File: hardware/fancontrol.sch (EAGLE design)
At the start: 7 parts, among them Q1 IRLZ44Z, T1 BC547

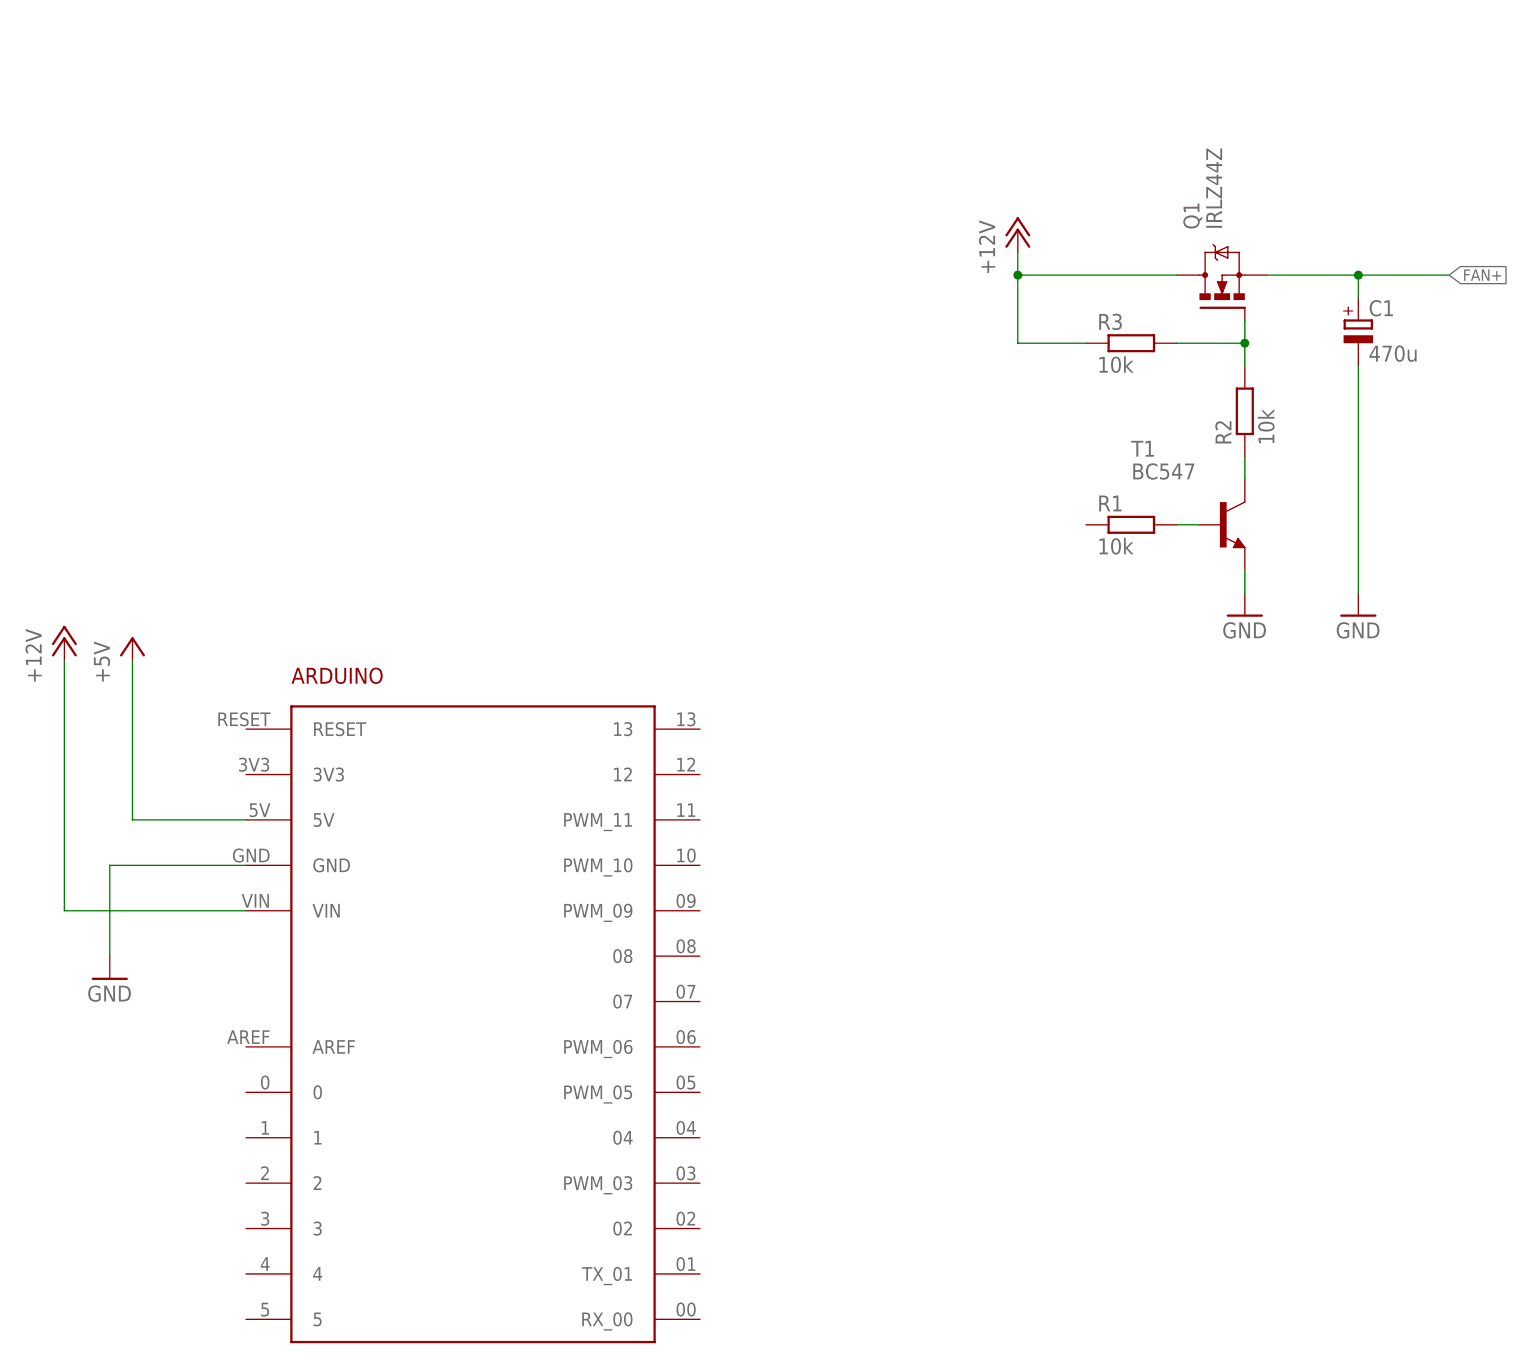
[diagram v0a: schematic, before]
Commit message: generated board
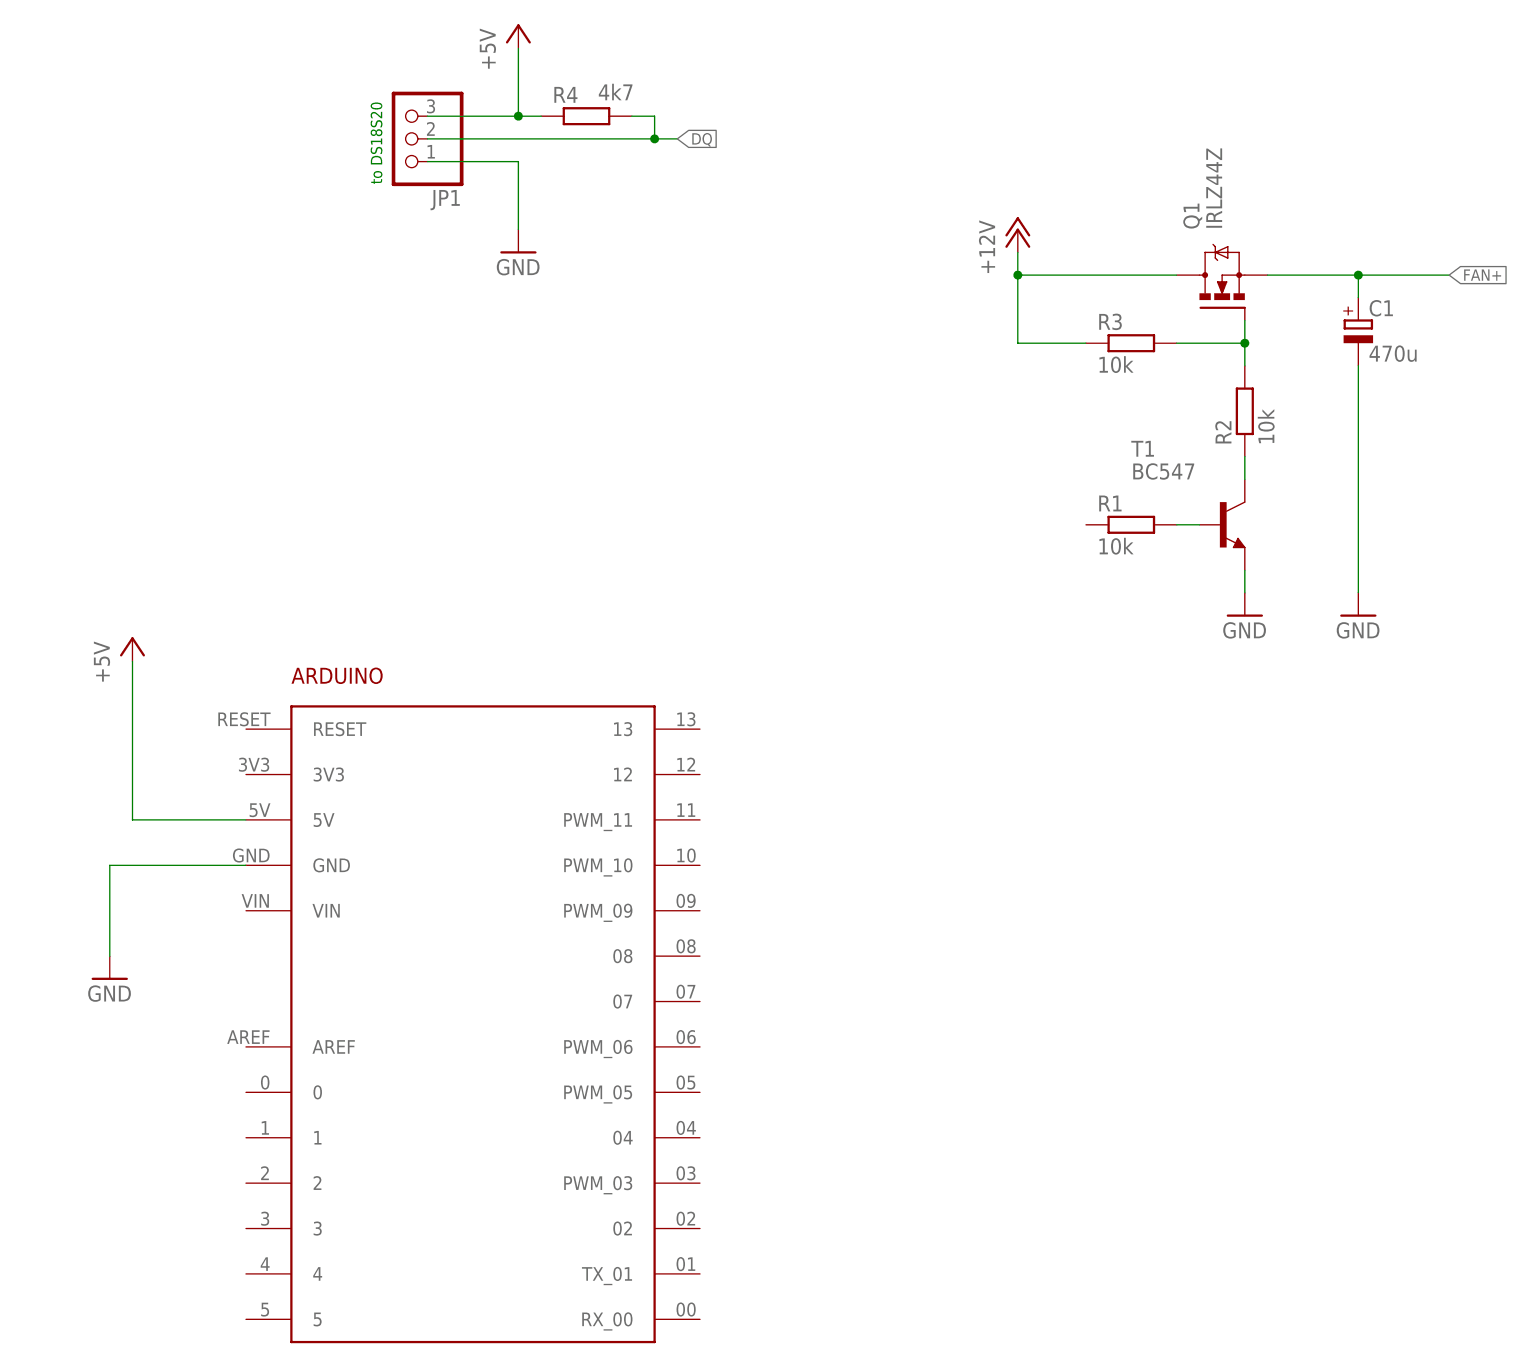
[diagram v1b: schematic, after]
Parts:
- added JP1: (no value), pinhead:PINHD-1X3
- added R4: 4k7, rcl:R-EU_0207/7
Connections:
- new net DQ: JP1.2, R4.2
- net +12V: no longer ARDUINO1.VIN
- net +5V: now also JP1.3, R4.1
- net GND: now also JP1.1
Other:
- note added: "to DS18S20"
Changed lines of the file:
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@@
 <part name="ARDUINO1" library="arduino" deviceset="ARDUINO" device=""/>
 <part name="GND3" library="supply1" deviceset="GND" device=""/>
-<part name="P+3" library="supply1" deviceset="+12V" device=""/>
 <part name="P+4" library="supply1" deviceset="+5V" device=""/>
+<part name="JP1" library="pinhead" deviceset="PINHD-1X3" device=""/>
+<part name="P+1" library="supply1" deviceset="+5V" device=""/>
+<part name="GND4" library="supply1" deviceset="GND" device=""/>
+<part name="R4" library="rcl" deviceset="R-EU_" device="0207/7" value="4k7"/>
 </parts>
 <sheets>
 <sheet>
 <plain>
+<text x="40.64" y="142.24" size="1.27" layer="91" rot="R90">to DS18S20</text>
 </plain>
 <instances>
@@
 <instance part="ARDUINO1" gate="G$1" x="50.8" y="50.8"/>
 <instance part="GND3" gate="1" x="10.16" y="53.34"/>
-<instance part="P+3" gate="1" x="5.08" y="91.44"/>
 <instance part="P+4" gate="1" x="12.7" y="91.44"/>
+<instance part="JP1" gate="A" x="43.18" y="147.32" rot="R180"/>
+<instance part="P+1" gate="1" x="55.88" y="160.02"/>
+<instance part="GND4" gate="1" x="55.88" y="134.62"/>
+<instance part="R4" gate="G$1" x="63.5" y="149.86" smashed="yes">
+<attribute name="NAME" x="59.69" y="151.3586" size="1.778" layer="95"/>
+<attribute name="VALUE" x="64.77" y="151.638" size="1.778" layer="96"/>
+</instance>
 </instances>
 <busses>
@@
 <wire x1="10.16" y1="66.04" x2="10.16" y2="55.88" width="0.1524" layer="91"/>
 </segment>
+<segment>
+<pinref part="JP1" gate="A" pin="1"/>
+<pinref part="GND4" gate="1" pin="GND"/>
+<wire x1="45.72" y1="144.78" x2="55.88" y2="144.78" width="0.1524" layer="91"/>
+<wire x1="55.88" y1="144.78" x2="55.88" y2="137.16" width="0.1524" layer="91"/>
+</segment>
 </net>
 <net name="N$3" class="0">
@@
 <junction x="111.76" y="132.08"/>
 </segment>
-<segment>
-<pinref part="ARDUINO1" gate="G$1" pin="VIN"/>
-<pinref part="P+3" gate="1" pin="+12V"/>
-<wire x1="25.4" y1="60.96" x2="5.08" y2="60.96" width="0.1524" layer="91"/>
-<wire x1="5.08" y1="60.96" x2="5.08" y2="88.9" width="0.1524" layer="91"/>
-</segment>
 </net>
 <net name="FAN+" class="0">
@@
 <wire x1="12.7" y1="71.12" x2="12.7" y2="88.9" width="0.1524" layer="91"/>
 </segment>
+<segment>
+<pinref part="JP1" gate="A" pin="3"/>
+<pinref part="R4" gate="G$1" pin="1"/>
+<wire x1="45.72" y1="149.86" x2="55.88" y2="149.86" width="0.1524" layer="91"/>
+<pinref part="P+1" gate="1" pin="+5V"/>
+<wire x1="55.88" y1="149.86" x2="58.42" y2="149.86" width="0.1524" layer="91"/>
+<wire x1="55.88" y1="157.48" x2="55.88" y2="149.86" width="0.1524" layer="91"/>
+<junction x="55.88" y="149.86"/>
+</segment>
 </net>
+<net name="DQ" class="0">
+<segment>
+<pinref part="JP1" gate="A" pin="2"/>
+<wire x1="45.72" y1="147.32" x2="71.12" y2="147.32" width="0.1524" layer="91"/>
+<label x="73.66" y="147.32" size="1.27" layer="95" xref="yes"/>
+<wire x1="71.12" y1="147.32" x2="73.66" y2="147.32" width="0.1524" layer="91"/>
+<wire x1="71.12" y1="149.86" x2="71.12" y2="147.32" width="0.1524" layer="91"/>
+<junction x="71.12" y="147.32"/>
+<pinref part="R4" gate="G$1" pin="2"/>
+<wire x1="68.58" y1="149.86" x2="71.12" y2="149.86" width="0.1524" layer="91"/>
+</segment>
+</net>
